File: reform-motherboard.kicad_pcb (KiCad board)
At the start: 4 copper layers, 130 x 99 mm, 210 parts, among them J1 TinyRex-J1-DF40C, J10 TEST_PMIC_ON, J11 TEST_ON, J12 USB_INT_3, J13 Conn_HDMI, J14 Conn_LVDS, J15 USB_INT_2, J16 Conn_LineIn, J17 Conn_LineOut, J18 TRRS, J19 Conn_BOOT, J2 TinyRex-J2-DF40C, J20 Conn_GPIO1, J21 Conn_01x06, J22 Conn_PWRON, J23 Conn_RESET, J24 Conn_01x04, J25 Conn_CONSOLE, J26 Conn_Backlight, J27 48099-5701, J28 Conn_SDWP, J29 Conn_5V, J3 TinyRex-J3-DF40C, J4 693072010801, J5 USB_A, J6 Barrel_Jack, J7 USB_A, J8 TEST_3V, J9 USB_INT_1, P1 5622-4100-ML, P2 J0G-0003NL, Q1 2N7002, Q4 Si5481DU, U1 MPCIE-Socket, U10 SGTL5000XNAA3, U11 LP3962EMP-2.5, U12 SN74LVC1G08DCKR, U13 TLV1117-15, U14 CM2020-00TR, U15 TPS2044BDR, U16 TUSB2046BVFR, U2 LTC4156IUFDPBF, U3 TPS61235RWLR, U4 AP1501A-33K5G-13, U5 74AHC1G14, U6 INA260AIPW, U7 LTC4415IMSEPBF, U8 INA260AIPW, Y1 6MHz

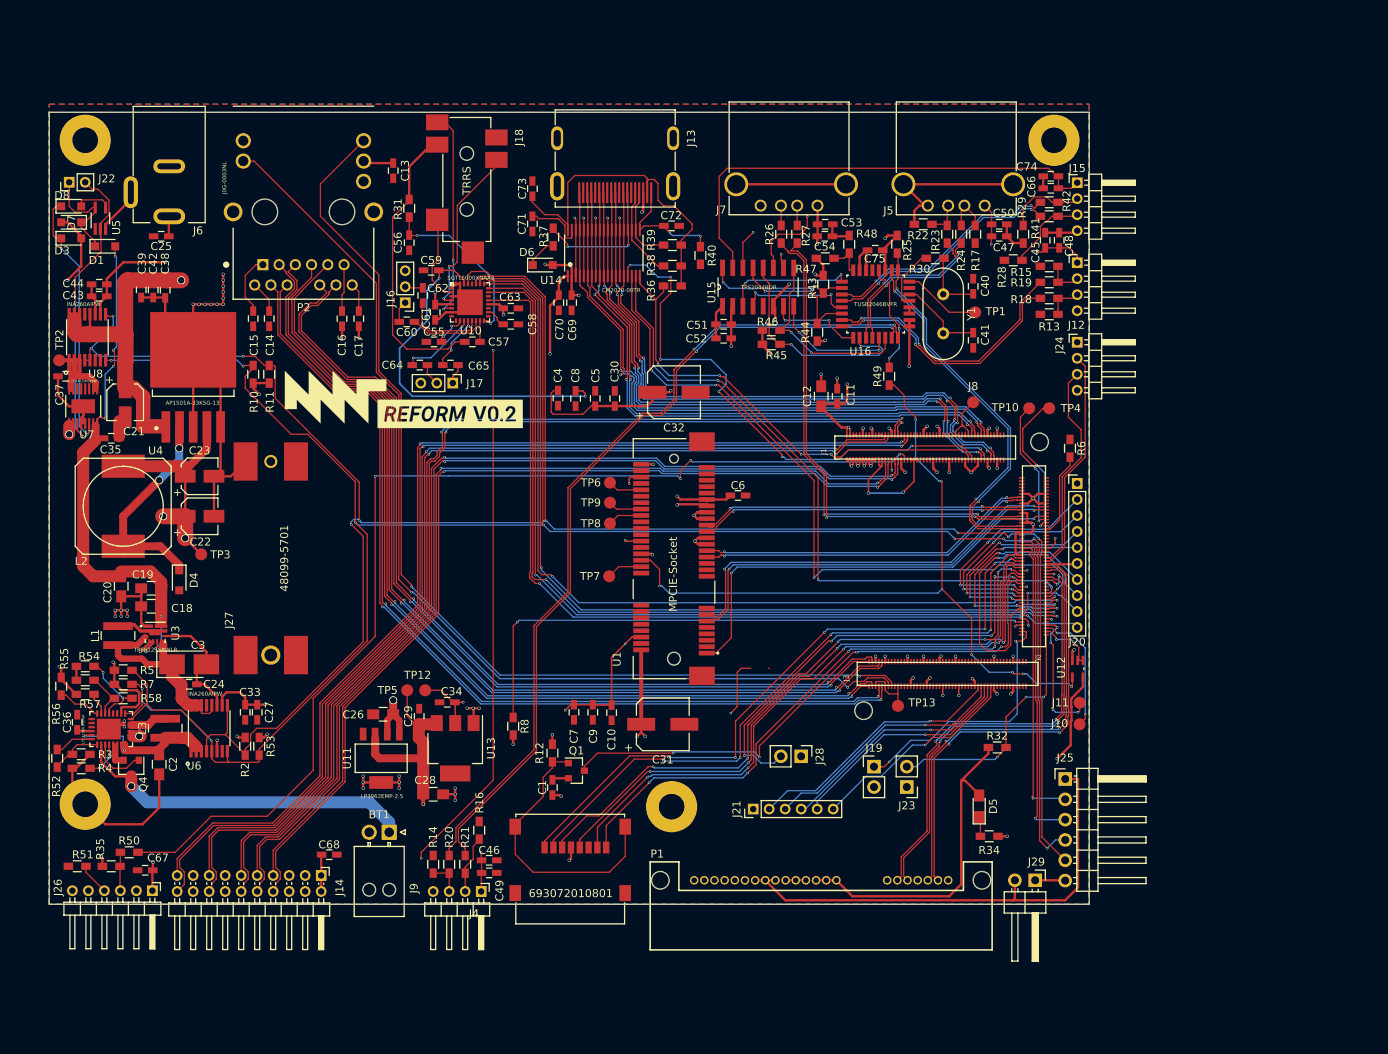
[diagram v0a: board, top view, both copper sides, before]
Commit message: motherboard 0.3 WIP snapshot schematics/PCB
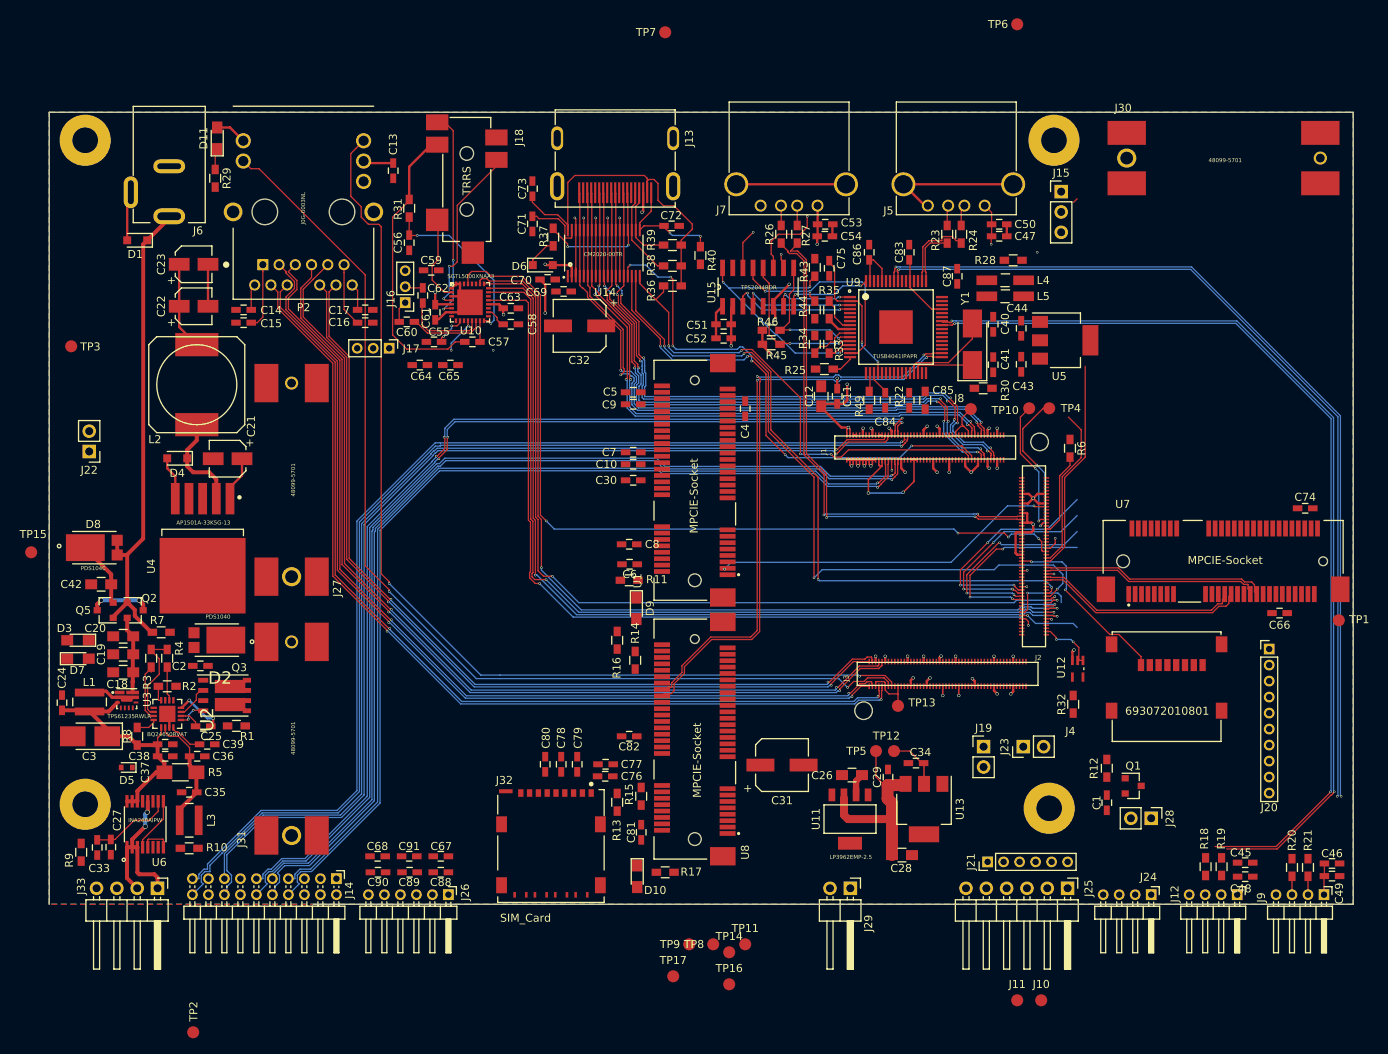
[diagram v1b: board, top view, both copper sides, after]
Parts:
- removed BT1: Molex 105313-1202, Connectors_Molex:Molex_NanoFit_1x02x2.50mm_Angled
- removed G***: LOGO, mnt:mnt
- removed G***: LOGO, mnt:reform02
- removed P1: 5622-4100-ML, 5622-4100-ML:3M_5622-4100-ML
- removed Q4: Si5481DU, TO_SOT_Packages_SMD:SOT-23
- removed R41, R42: 27, Resistors_SMD:R_0603_HandSoldering
- removed R47, R48, R56, R58: 0, Resistors_SMD:R_0603_HandSoldering
- removed R50, R51: R0, Resistors_SMD:R_0603_HandSoldering
- removed R52: 100k, Resistors_SMD:R_0603_HandSoldering
- removed R53: 4.7k, Resistors_SMD:R_0603_HandSoldering
- removed R54, R55: 1.21k, Resistors_SMD:R_0603_HandSoldering
- removed R57: 3.6k, Resistors_SMD:R_0603_HandSoldering
- removed U16: TUSB2046BVFR, TUSB2046BVFR:QFP80P900X900X145-32N
- added C76: 10uF, Capacitors_SMD:C_0603_HandSoldering, F.Cu at (99.5, 104.0)
- added C77: 0.1uF, Capacitors_SMD:C_0603_HandSoldering, F.Cu at (99.5, 102.5)
- added C78: 33pF, Capacitors_SMD:C_0603_HandSoldering, F.Cu at (94.0, 102.5)
- added C79: 33pF, Capacitors_SMD:C_0603_HandSoldering, F.Cu at (96.0, 102.5)
- added C80: 33pF, Capacitors_SMD:C_0603_HandSoldering, F.Cu at (92.0, 102.5)
- added C81: 0.1uF, Capacitors_SMD:C_0603_HandSoldering, F.Cu at (104.0, 111.0)
- added C82: 10uF, Capacitors_SMD:C_0603_HandSoldering, F.Cu at (102.5, 99.0)
- added C83: 0.1uF, Capacitors_SMD:C_0603_HandSoldering, F.Cu at (137.5, 38.5)
- added C84: 0.1uF, Capacitors_SMD:C_0603_HandSoldering, F.Cu at (134.5, 57.0)
- added C85: 10uF, Capacitors_SMD:C_0603_HandSoldering, F.Cu at (137.5, 57.0)
- added C86: 0.1uF, Capacitors_SMD:C_0603_HandSoldering, F.Cu at (132.5, 38.5)
- added C87: 0.1uF, Capacitors_SMD:C_0603_HandSoldering, F.Cu at (143.5, 41.5)
- added C88: 0.1uF, Capacitors_SMD:C_0603_HandSoldering, F.Cu at (79.0, 116.0)
- added C89: 10uF, Capacitors_SMD:C_0603_HandSoldering, F.Cu at (75.0, 116.0)
- added C90: 0.1uF, Capacitors_SMD:C_0603_HandSoldering, F.Cu at (71.1, 116.0)
- added C91: 0.1uF, Capacitors_SMD:C_0603_HandSoldering, F.Cu at (75.0, 114.0)
- added D10: LED_WWAN, LEDs:LED_0805_HandSoldering, F.Cu at (103.5, 116.5)
- added D11: LED_3V3, LEDs:LED_0805_HandSoldering, F.Cu at (51.0, 24.2)
- added D2: PDS1040, PDS1040:DIO_SBR10U200P5-13, F.Cu at (51.0, 87.0)
- added D9: LED_WLAN, LEDs:LED_0805_HandSoldering, F.Cu at (103.4, 83.0)
- added J30: 48099-5701, 48099-5701:MOLEX_48099-5701, F.Cu at (176.8, 26.7)
- added J31: 48099-5701, 48099-5701:MOLEX_48099-5701, F.Cu at (60.3, 99.3)
- added J32: SIM_Card, TE-2199337-5:TE_2199337-5, F.Cu at (92.7, 112.7)
- added J33: BAT, Pin_Headers:Pin_Header_Angled_1x04_Pitch2.54mm, F.Cu at (43.5, 118.0)
- added L4: 220@100MHz, Choke_SMD:Choke_SMD_1206_Handsoldering, F.Cu at (149.5, 42.0)
- added L5: 220@100MHz, Choke_SMD:Choke_SMD_1206_Handsoldering, F.Cu at (149.5, 44.0)
- added Q2: Si2333DDS, TO_SOT_Packages_SMD:SOT-23, F.Cu at (40.8, 83.2)
- added Q3: Si7288DP, Housings_SOIC:PowerPAK_SO-8_Dual, F.Cu at (51.9, 93.9)
- added Q5: Si2333DDS, TO_SOT_Packages_SMD:SOT-23, F.Cu at (37.0, 83.2)
- added R1: 100k, Resistors_SMD:R_0603_HandSoldering, F.Cu at (53.4, 97.7)
- added R33: 4.7k, Resistors_SMD:R_0603_HandSoldering, F.Cu at (127.5, 50.0)
- added R9: 330, Resistors_SMD:R_0603_HandSoldering, F.Cu at (34.0, 113.5)
- added TP11: WWAN_UART_TX, Measurement_Points:Measurement_Point_Round-SMD-Pad_Small, F.Cu at (117.0, 125.0)
- added TP14: WWAN_UART_RX, Measurement_Points:Measurement_Point_Round-SMD-Pad_Small, F.Cu at (115.0, 126.0)
- added TP15: TEST_5V, Measurement_Points:Measurement_Point_Round-SMD-Pad_Small, F.Cu at (27.8, 76.0)
- added TP16: WWAN_WAKE_OUT, Measurement_Points:Measurement_Point_Round-SMD-Pad_Small, F.Cu at (115.0, 130.0)
- added TP17: WWAN_RFKILL, Measurement_Points:Measurement_Point_Round-SMD-Pad_Small, F.Cu at (108.0, 129.0)
- added U9: TUSB4041IPAPR, TUSB4041IPAPR:QFP50P1200X1200X105-65N, F.Cu at (135.8, 47.9)
- C2: value 22uF -> 1uF; footprint Capacitors_SMD:C_0805_HandSoldering -> Capacitors_SMD:C_0603_HandSoldering
- C25, C66: value 10uF -> 0.1uF
- C35, C37: value 4.7uF -> 0.1uF
- C36: value 0.047uF -> 0.1uF
- C40, C41: value 27pF -> 18pF
- C42: value 0.1uF -> 100uF; footprint Capacitors_SMD:C_0603_HandSoldering -> Capacitors_SMD:C_0805_HandSoldering
- C43: value 10uF -> 1uF
- C44: value 0.1uF -> 1uF
- C45, C46, C47, C53: value 10uF -> 22uF
- C74: value 0.1uF -> 10uF
- D1: value D_Schottky -> D_Zener
- D3: value D -> LED_CStat2; footprint Diodes_SMD:D_SOD-323_HandSoldering -> LEDs:LED_0805_HandSoldering
- D5: value LED_3V3 -> ZLLS350; footprint LEDs:LED_0805_HandSoldering -> Diodes_SMD:D_SOD-523
- D7: value D_Schottky -> LED_Charge; footprint Diodes_SMD:D_SOD-323_HandSoldering -> LEDs:LED_0805_HandSoldering
- D8: value D -> PDS1040; footprint Diodes_SMD:D_SOD-323_HandSoldering -> PDS1040:DIO_SBR10U200P5-13
- J15: value USB_INT_2 -> Conn_01x03; footprint Pin_Headers:Pin_Header_Angled_1x04_Pitch2.00mm -> Pin_Headers:Pin_Header_Straight_1x03_Pitch2.54mm
- J22: value Conn_PWRON -> Conn_01x02; footprint Pin_Headers:Pin_Header_Straight_1x02_Pitch2.00mm -> Pin_Headers:Pin_Header_Straight_1x02_Pitch2.54mm
- L3: value 1 uH -> 10 uH
- R11: value 4.7k -> 240
- R13, R14, R15, R16: value 15k -> 0
- R17, R29: value 15k -> 240
- R2: value 4.7k -> 100k
- R22: value 15k -> 9.53k
- R25: value 1.5k -> 10k
- R28: value 15k -> 90.9k
- R3: value 100k -> 0
- R30: value 1.5k -> 1M
- R34: value 240 -> 4.7k
- R35: value R0 -> 4.7k
- R4: value 499 -> 0
- R5: value 4.7k -> 20m; footprint Resistors_SMD:R_0603_HandSoldering -> Resistors_SMD:R_1206_HandSoldering
- R7: value 4.7k -> 330
- R8: value 0 -> 3.6k
- TP1: value TEST_USB_SUSP -> SATA_DA
- TP2: value TEST_5V -> TEST_BATOUT
- TP6: value PCIe_WLANn -> TEST_1V1
- TP8: value PCIe_USB_D- -> UIM_C4
- TP9: value PCIe_USB_D+ -> UIM_C8
- U2: value LTC4156IUFDPBF -> BQ24650RVAT; footprint LTC4156-Custom:QFN-28_UFD -> BQ24650RVAT:QFN50P350X350X100-17N
- U5: value 74AHC1G14 -> TLV74311PDBVR; footprint TO_SOT_Packages_SMD:SOT-353_SC-70-5_Handsoldering -> TO_SOT_Packages_SMD:SOT-223
- U7: value LTC4415IMSEPBF -> MPCIE-Socket; footprint LTC4415IMSEPBF:MSOP-16_MSE -> 67910-5700:MOLEX_67910-5700
- U8: value INA260AIPW -> MPCIE-Socket; footprint INA260AIPW:SOP65P640X120-16N -> 67910-5700:MOLEX_67910-5700
- Y1: value 6MHz -> 24MHz; footprint Crystals:Crystal_HC49-4H_Vertical -> Crystals:Crystal_SMD_5032-2pin_5.0x3.2mm_HandSoldering
- moved U7 142.0 mm to (174.9, 77.1), turned to 0 degrees
- moved U5 121.6 mm to (157.0, 49.5), turned to 0 degrees
- moved C43 115.6 mm to (151.5, 52.5), turned to 270 degrees
- moved C44 115.4 mm to (151.5, 48.0), turned to 90 degrees
- moved R35 113.5 mm to (127.5, 45.7), turned to 270 degrees
- moved D5 106.7 mm to (39.7, 102.9), turned to 180 degrees
- moved C46 105.4 mm to (190.3, 114.9)
- moved C49 105.4 mm to (190.3, 116.5)
- moved J9 105.4 mm to (189.3, 118.8)
- moved R20 105.4 mm to (185.3, 115.4)
- moved R21 105.4 mm to (187.3, 115.4)
- moved R29 101.2 mm to (50.8, 29.2)
- moved U8 92.0 mm to (110.7, 101.2)
- moved R17 88.7 mm to (107.0, 116.0), turned to 180 degrees
- moved TP2 85.7 mm to (48.0, 136.0)
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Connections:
- net Net-(J2-Pad10) renamed GPIO3
- C2 pad 1: Net-(C2-Pad1) -> CHGVCC
- C25 pad 2: GND -> Net-(C25-Pad2)
- C27 pad 1: +3V3 -> Net-(C27-Pad1)
- C33 pad 1: +3V3 -> Net-(C27-Pad1)
- C35 pad 1: Net-(C18-Pad1) -> Net-(C35-Pad1)
- C35 pad 2: GND -> Net-(C24-Pad1)
- C36 pad 1: Net-(C36-Pad1) -> Net-(C35-Pad1)
- C37 pad 1: Net-(C37-Pad1) -> Net-(C24-Pad1)
- C38 pad 1: +5V -> Net-(C24-Pad1)
- C39 pad 1: +5V -> Net-(C39-Pad1)
- C42 pad 1: +5V -> Net-(C42-Pad1)
- C43 pad 1: +3V3 -> POK_1V5
- C44 pad 1: +3V3 -> +1V1
- C66 pad 1: USB_HUB0_5V -> +3V3
- C67 pad 1: +5V -> GND
- C67 pad 2: GND -> +5V
- C68 pad 1: +3V3 -> GND
- C68 pad 2: GND -> +3V3
- C74 pad 1: USB_HUB0_5V -> +3V3
- C75 pad 1: +3V3 -> Net-(C75-Pad1)
- D1 pad 1: Net-(D1-Pad1) -> CHGVCC
- D1 pad 2: Net-(C18-Pad1) -> GND
- D3 pad 1: BATOFF -> Net-(D3-Pad1)
- D3 pad 2: Net-(C25-Pad1) -> Net-(D3-Pad2)
- D5 pad 1: Net-(D5-Pad1) -> Net-(C25-Pad1)
- D5 pad 2: +3V3 -> Net-(C39-Pad1)
- D7 pad 1: Net-(D1-Pad1) -> Net-(D7-Pad1)
- D7 pad 2: Net-(C25-Pad1) -> Net-(D7-Pad2)
- D8 pad 1: BATOFF -> Net-(C42-Pad1)
- D8 pad 2: Net-(D8-Pad2) -> CHGVCC
- J1 pad 38: LVDS0_PWM -> GPIO2
- J14 pad 4: Net-(J14-Pad4) -> +3V3
- J15 pad 1: USB_HUB0_5V -> +5V
- J15 pad 2: Net-(J15-Pad2) -> FAN_PWM
- J15 pad 3: Net-(J15-Pad3) -> GND
- J2 pad 17: Net-(J2-Pad17) -> LVDS0_PWM
- J2 pad 19: Net-(J2-Pad19) -> FAN_PWM
- J2 pad 66: Net-(J2-Pad66) -> GND
- J2 pad 68: Net-(J2-Pad66) -> Net-(J2-Pad68)
- J2 pad 7: +5V -> POK_5V
- J20 pad 7: Net-(J2-Pad19) -> Net-(J20-Pad7)
- J20 pad 8: Net-(J2-Pad17) -> Net-(J20-Pad8)
- J22 pad 1: Net-(D1-Pad1) -> +5V
- J22 pad 2: PWRON -> Net-(C42-Pad1)
- J26 pad 3: Net-(J26-Pad3) -> +3V3
- J26 pad 4: Net-(J26-Pad4) -> LVDS0_PWM
- J6 pad 1: Net-(C25-Pad1) -> CHGVCC
- L3 pad 1: Net-(C2-Pad1) -> Net-(C25-Pad2)
- L3 pad 2: Net-(L3-Pad2) -> Net-(C35-Pad1)
- R10 pad 1: I2C3_SDA -> GND
- R10 pad 2: +3V3 -> Net-(C24-Pad1)
- R11 pad 2: I2C3_SCL -> Net-(D9-Pad2)
- R13 pad 1: GND -> Net-(C76-Pad2)
- R13 pad 2: Net-(J12-Pad3) -> UIM_PWR
- R14 pad 2: Net-(J9-Pad3) -> UIM_DET
- R15 pad 1: Net-(J12-Pad2) -> Net-(J32-Pad6)
- R15 pad 2: GND -> UIM_VPP
- R16 pad 1: Net-(J9-Pad2) -> RESETn
- R16 pad 2: GND -> Net-(R16-Pad2)
- R17 pad 1: GND -> +3V3
- R17 pad 2: Net-(J5-Pad2) -> Net-(D10-Pad2)
- R2 pad 1: +3V3 -> Net-(R2-Pad1)
- R2 pad 2: I2C3_SCL -> GND
- R22 pad 1: Net-(J5-Pad3) -> GND
- R22 pad 2: GND -> Net-(R22-Pad2)
- R25 pad 1: +3V3 -> GND
- R25 pad 2: USB1_P -> Net-(R25-Pad2)
- R28 pad 1: GND -> +5V
- R28 pad 2: Net-(J15-Pad3) -> Net-(R25-Pad2)
- R29 pad 1: Net-(J15-Pad2) -> Net-(D11-Pad1)
- R3 pad 1: GND -> Net-(R3-Pad1)
- R30 pad 1: Net-(R30-Pad1) -> Net-(C40-Pad1)
- R30 pad 2: Net-(C40-Pad1) -> Net-(C41-Pad1)
- R34 pad 1: Net-(D5-Pad1) -> Net-(R34-Pad1)
- R35 pad 1: Net-(J26-Pad3) -> Net-(R35-Pad1)
- R35 pad 2: +3V3 -> GND
- R4 pad 1: GND -> Net-(R4-Pad1)
- R4 pad 2: Net-(R4-Pad2) -> Net-(R3-Pad2)
- R49 pad 1: RESETn -> Net-(R49-Pad1)
- R49 pad 2: Net-(R49-Pad2) -> RESETn
- R5 pad 1: I2C3_SCL -> Net-(C35-Pad1)
- R5 pad 2: +3V3 -> Net-(C24-Pad1)
- R6 pad 2: Net-(J2-Pad66) -> Net-(J2-Pad68)
- R7 pad 1: +3V3 -> CHGVCC
- R7 pad 2: I2C3_SDA -> Net-(D3-Pad2)
- R8 pad 1: POK_3V3 -> Net-(C24-Pad1)
- R8 pad 2: +3V3 -> Net-(R8-Pad2)
- TP2 pad 1: Net-(C37-Pad1) -> Net-(C24-Pad1)
- TP6 pad 1: Net-(TP6-Pad1) -> +1V1
- U1 pad 36: Net-(TP8-Pad1) -> Net-(U1-Pad36)
- U1 pad 38: Net-(TP9-Pad1) -> Net-(U1-Pad38)
- U1 pad 44: Net-(TP6-Pad1) -> Net-(D9-Pad1)
- U11 pad 1: +3V3 -> PWRON
- U2 pad 1: I2C3_SDA -> CHGVCC
- U2 pad 10: Net-(U2-Pad10) -> Net-(C35-Pad1)
- U2 pad 11: Net-(U2-Pad11) -> GND
- U2 pad 12: Net-(C36-Pad1) -> Net-(C39-Pad1)
- U2 pad 13: Net-(C2-Pad1) -> Net-(Q3-Pad4)
- U2 pad 14: Net-(R52-Pad2) -> Net-(C25-Pad2)
- U2 pad 15: Net-(R3-Pad2) -> Net-(Q3-Pad2)
- U2 pad 16: Net-(BT1-Pad1) -> Net-(C25-Pad1)
- U2 pad 17: Net-(Q4-Pad1) -> GND
- U2 pad 2: +3V3 -> Net-(R4-Pad1)
- U2 pad 3: Net-(U2-Pad3) -> Net-(D7-Pad1)
- U2 pad 4: Net-(U2-Pad4) -> Net-(R2-Pad1)
- U2 pad 5: Net-(R54-Pad2) -> Net-(D3-Pad1)
- U2 pad 6: Net-(R55-Pad1) -> Net-(R3-Pad2)
- U2 pad 7: Net-(R57-Pad1) -> Net-(R3-Pad1)
- U2 pad 8: Net-(R56-Pad1) -> Net-(R8-Pad2)
- U2 pad 9: Net-(U2-Pad9) -> Net-(C24-Pad1)
- U3 pad 7: Net-(C24-Pad1) -> PWRON
- U5 pad 1: (no net) -> GND
- U5 pad 2: PWRON -> +1V1
- U5 pad 3: GND -> POK_1V5
- U5 pad 4: Net-(D8-Pad2) -> (no net)
- U6 pad 1: Net-(C2-Pad1) -> BATVCC
- U6 pad 10: +3V3 -> Net-(C27-Pad1)
- U6 pad 12: Net-(C24-Pad1) -> BATVCC
- U6 pad 2: Net-(C2-Pad1) -> BATVCC
- U6 pad 3: Net-(C2-Pad1) -> BATVCC
- U7 pad 1: Net-(C25-Pad1) -> Net-(U7-Pad1)
- U7 pad 10: Net-(C37-Pad1) -> Net-(U7-Pad10)
- U7 pad 15: Net-(C37-Pad1) -> GND
- U7 pad 16: Net-(C37-Pad1) -> Net-(U7-Pad16)
- U7 pad 17: GND -> Net-(U7-Pad17)
- U7 pad 2: Net-(C25-Pad1) -> +3V3
- U7 pad 3: PWRON -> Net-(U7-Pad3)
- U7 pad 4: GND -> Net-(U7-Pad4)
- U7 pad 5: GND -> Net-(U7-Pad5)
- U7 pad 6: BATOFF -> Net-(U7-Pad6)
- U7 pad 7: Net-(C18-Pad1) -> Net-(U7-Pad7)
- U7 pad 8: Net-(C18-Pad1) -> Net-(U7-Pad8)
- U7 pad 9: Net-(C37-Pad1) -> Net-(U7-Pad9)
- U8 pad 1: Net-(C37-Pad1) -> Net-(TP16-Pad1)
- U8 pad 10: +3V3 -> UIM_DATA
- U8 pad 11: GND -> Net-(TP14-Pad1)
- U8 pad 12: +5V -> UIM_CLK
- U8 pad 14: +5V -> UIM_RST
- U8 pad 15: +5V -> GND
- U8 pad 16: +5V -> UIM_VPP
- U8 pad 2: Net-(C37-Pad1) -> +3V3
- U8 pad 3: Net-(C37-Pad1) -> Net-(U8-Pad3)
- U8 pad 4: I2C3_SCL -> GND
- U8 pad 5: I2C3_SCL -> Net-(U8-Pad5)
- U8 pad 6: GND -> POK_1V5
- U8 pad 8: I2C3_SDA -> UIM_PWR
- U8 pad 9: I2C3_SCL -> GND
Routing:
- net +5V: track 426.8 -> 112.8 mm, vias 15 -> 12
- net I2C3_SDA: track 237.6 -> 3.88 mm, vias 9 -> 0
- net +3V3: track 241.3 -> 51.8 mm, vias 33 -> 6
- net GND: track 352.6 -> 169.7 mm, vias 83 -> 43
- net I2C3_SCL: track 252.7 -> 112.0 mm, vias 9 -> 4
- net LVDS0_PWM: track 135.0 -> 0.00 mm, vias 4 -> 0
- net POK_1V5: track 121.6 -> 6.94 mm, vias 7 -> 0
- net Net-(C25-Pad1): track 105.9 -> 6.48 mm, vias 4 -> 2
- net RESETn: track 94.6 -> 0.00 mm, vias 8 -> 0
- net USB_HUB1_P: track 32.5 -> 117.6 mm
- net USB_HUB1_N: track 33.2 -> 117.5 mm
- net SD3_DATA3: track 81.1 -> 0.00 mm, vias 4 -> 0
- net SD3_CMD: track 79.8 -> 0.00 mm, vias 6 -> 0
- net USB_HUB3_5V: track 125.3 -> 46.9 mm, vias 4 -> 2
- net POK_2V5: track 107.7 -> 29.7 mm, vias 3 -> 2
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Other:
- board size 130 x 99 mm -> 163 x 99 mm
- net class PWRFAT added: clearance 0.15, trace_width 0.5, via_dia 0.6, via_drill 0.5
